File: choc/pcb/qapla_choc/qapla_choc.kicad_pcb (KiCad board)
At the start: 2 copper layers, 154.4 x 126.1 mm, 72 parts

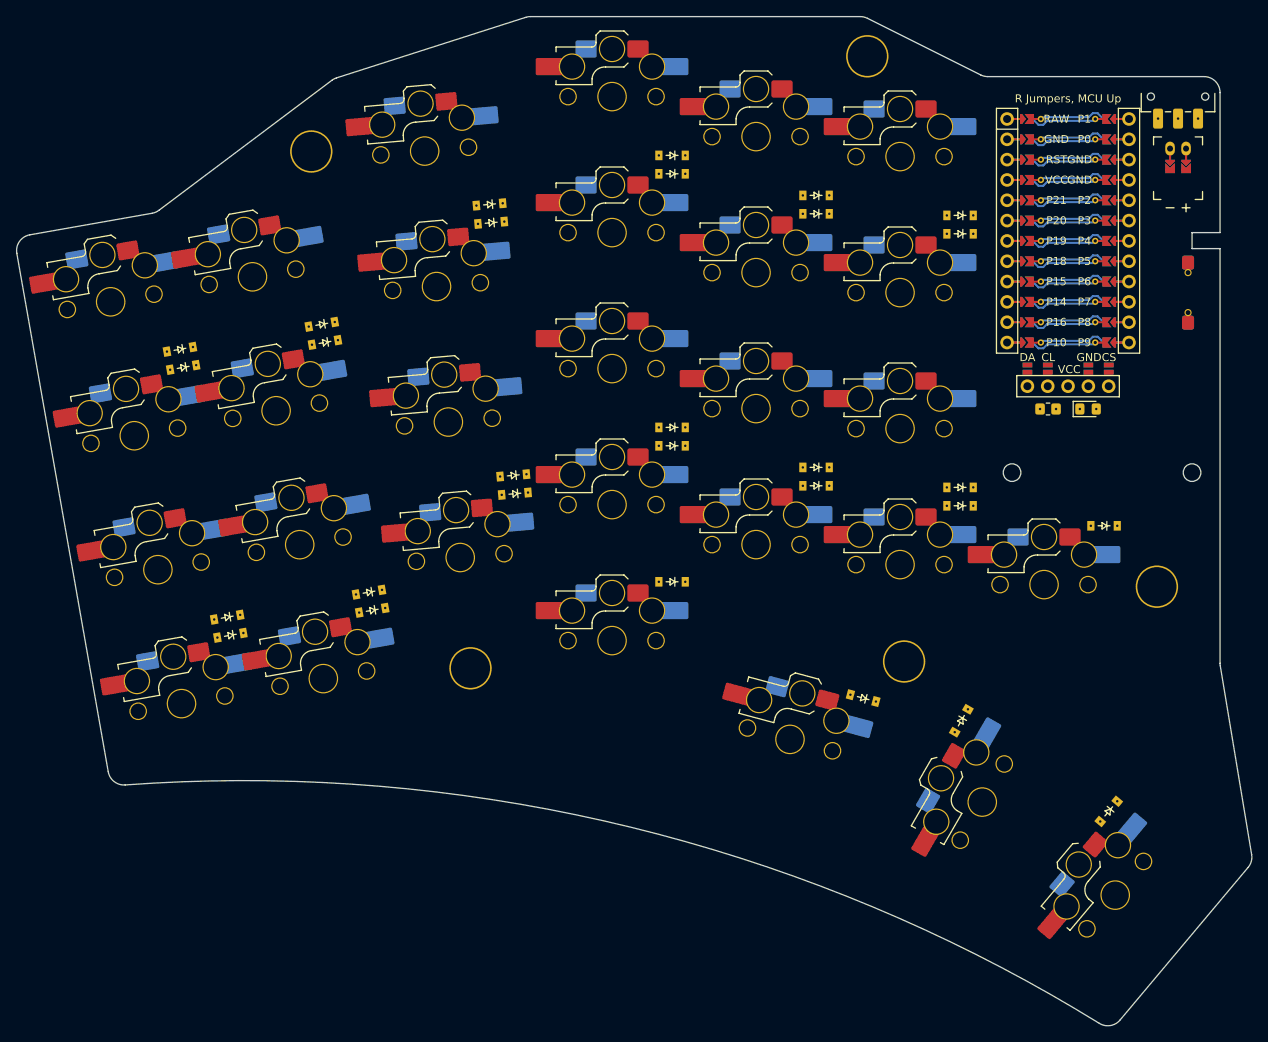
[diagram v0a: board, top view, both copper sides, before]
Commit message: Finalize choc case and pcb design
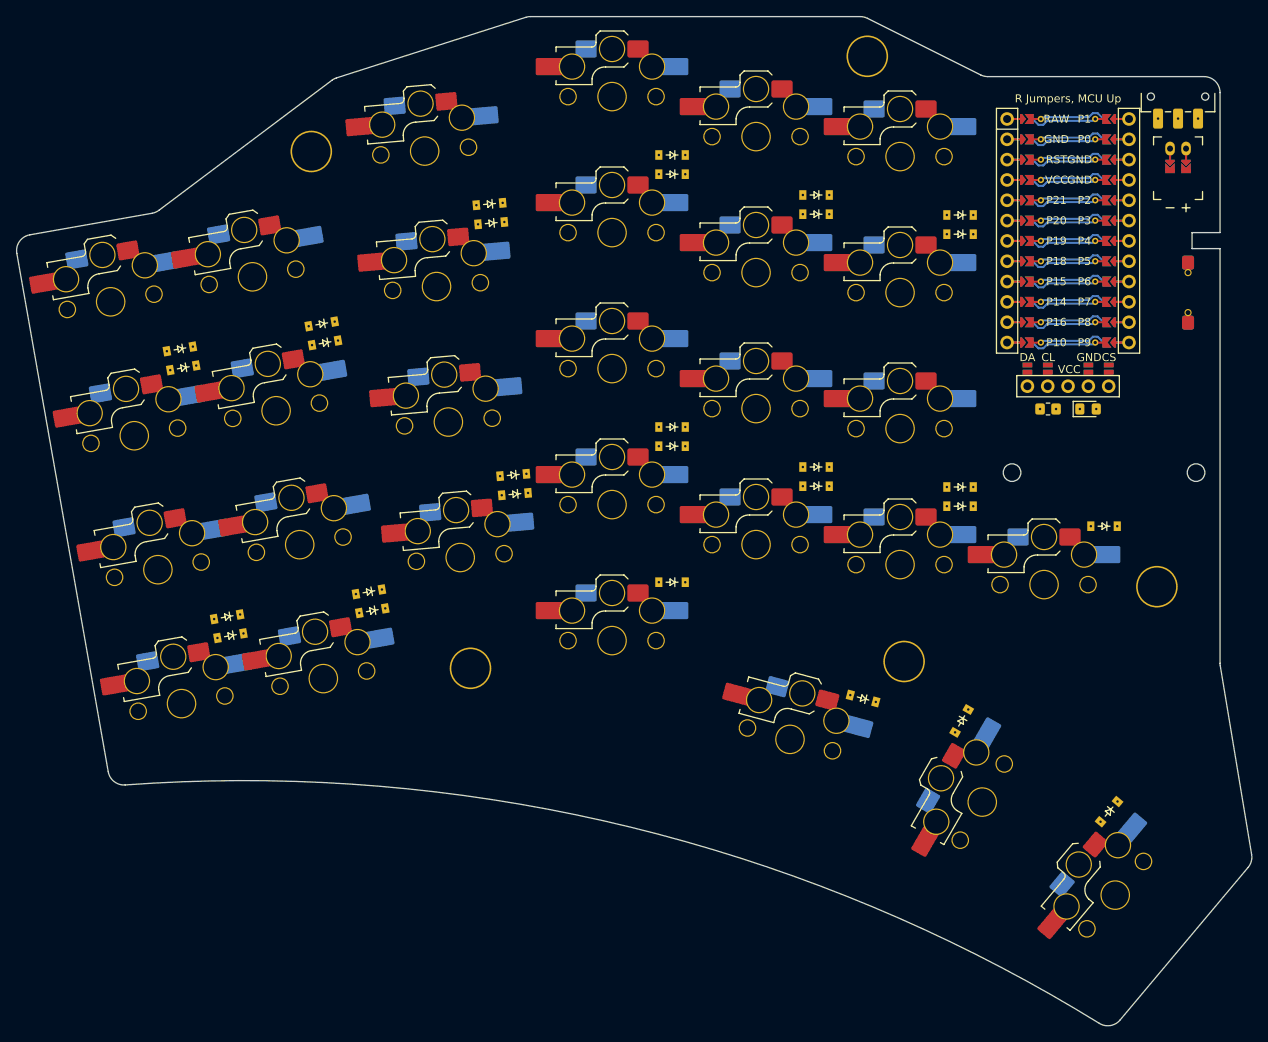
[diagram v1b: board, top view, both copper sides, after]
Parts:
- moved MH2 0.50 mm to (248.4, 84.7)
- moved D5 0.05 mm to (163.0, 85.0)
- moved D6 0.05 mm to (160.1, 51.2)
- moved D1 0.05 mm to (127.3, 102.8)
- moved D2 0.05 mm to (121.4, 69.3)
- moved D13 0.05 mm to (127.7, 105.1)
- moved D14 0.05 mm to (121.8, 71.6)
- moved D15 0.05 mm to (145.4, 102.0)
- moved D16 0.05 mm to (139.5, 68.5)
- moved D3 0.05 mm to (145.0, 99.6)
- moved D4 0.05 mm to (139.1, 66.2)
- moved D28 0.05 mm to (219.1, 115.8)
- moved D27 0.05 mm to (206.8, 113.0)
- moved D10 0.05 mm to (200.9, 50.0)
- moved D12 0.05 mm to (218.9, 52.5)
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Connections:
- _3 pad 3: GND -> P4
